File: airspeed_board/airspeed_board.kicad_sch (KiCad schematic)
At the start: 6 parts, among them J1 BME280, J2 ADXL345, J3 MPXV5002DP, U1 ESP32-C3_SUPERMINI, U2 XGZP6897D_1, U3 XGZP6897D_2

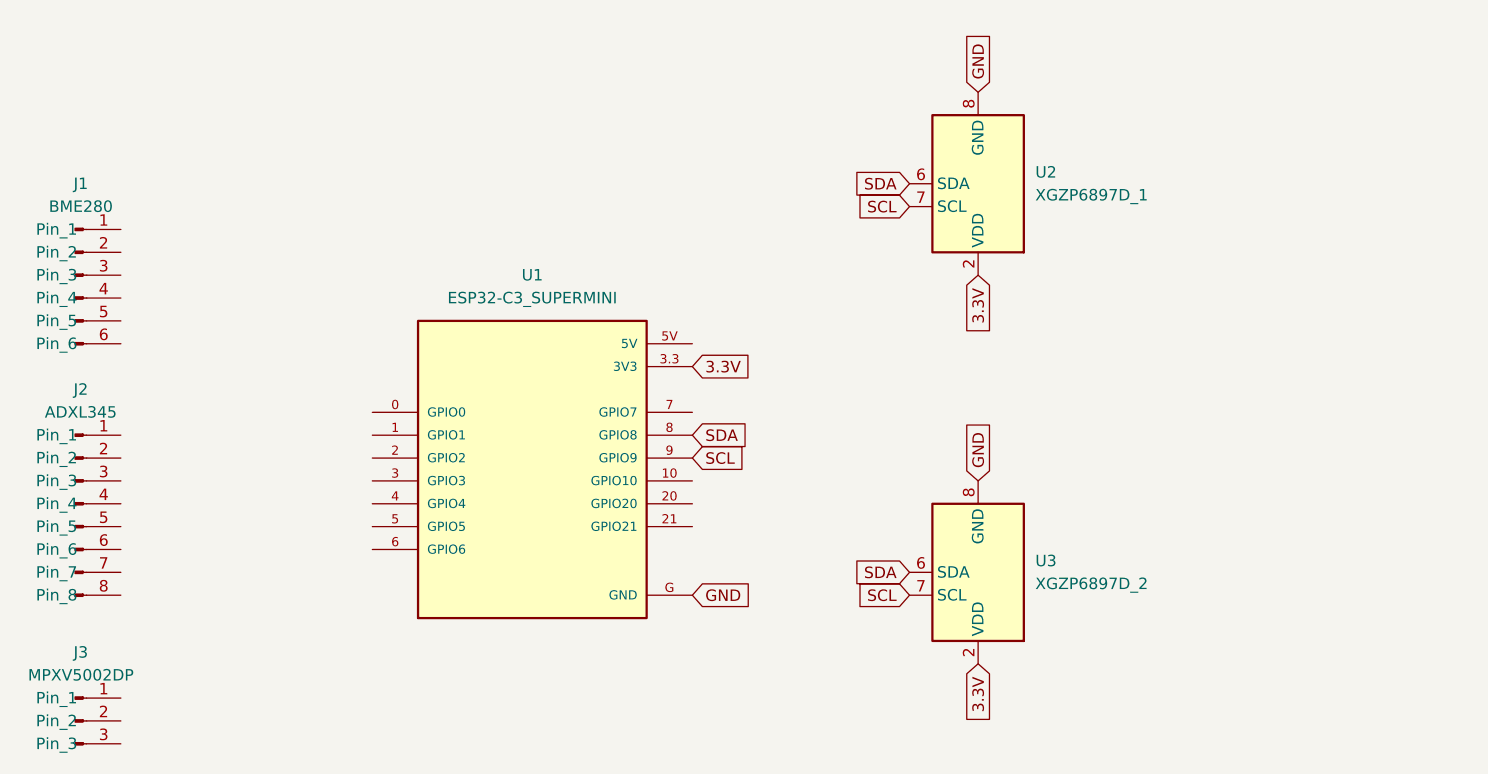
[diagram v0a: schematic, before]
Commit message: updated board layout
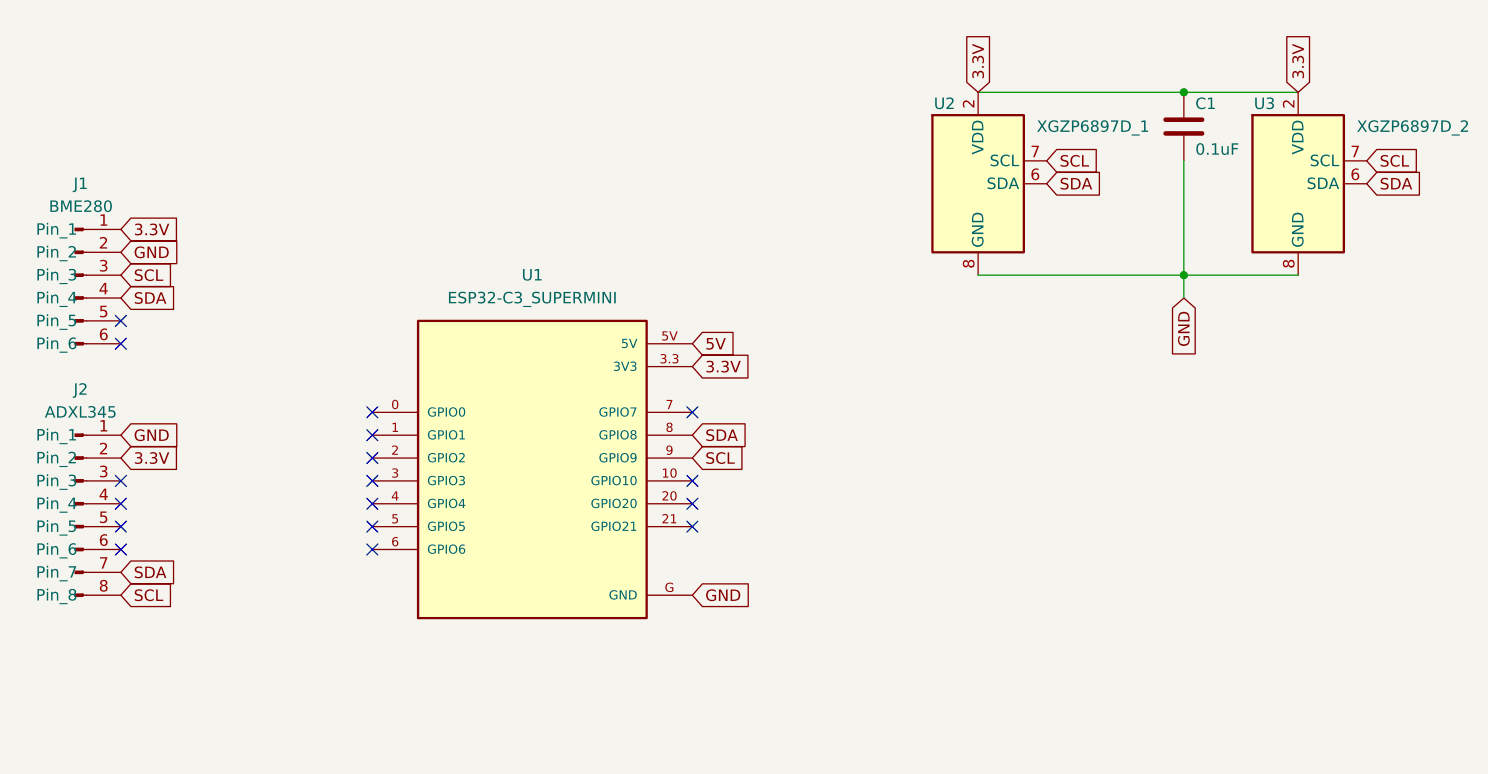
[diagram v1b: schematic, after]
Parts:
- removed J3: MPXV5002DP, Connector_PinHeader_2.54mm:PinHeader_1x03_P2.54mm_Vertical, symbol Connector:Conn_01x03_Pin
- added C1: 0.1uF, Capacitor_SMD:C_0805_2012Metric, symbol Device:C
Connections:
- net 3.3V: now also J1.1 (Pin_1), J2.2 (Pin_2), C1.2
- net GND: now also J1.2 (Pin_2), J2.1 (Pin_1), C1.1
- net SCL: now also J1.3 (Pin_3), J2.8 (Pin_8)
- net SDA: now also J1.4 (Pin_4), J2.7 (Pin_7)
- net 5V: now reaches U1.5V
- no-connect marks 0 -> 17
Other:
- moved on the sheet: U2

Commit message: updates to pcb
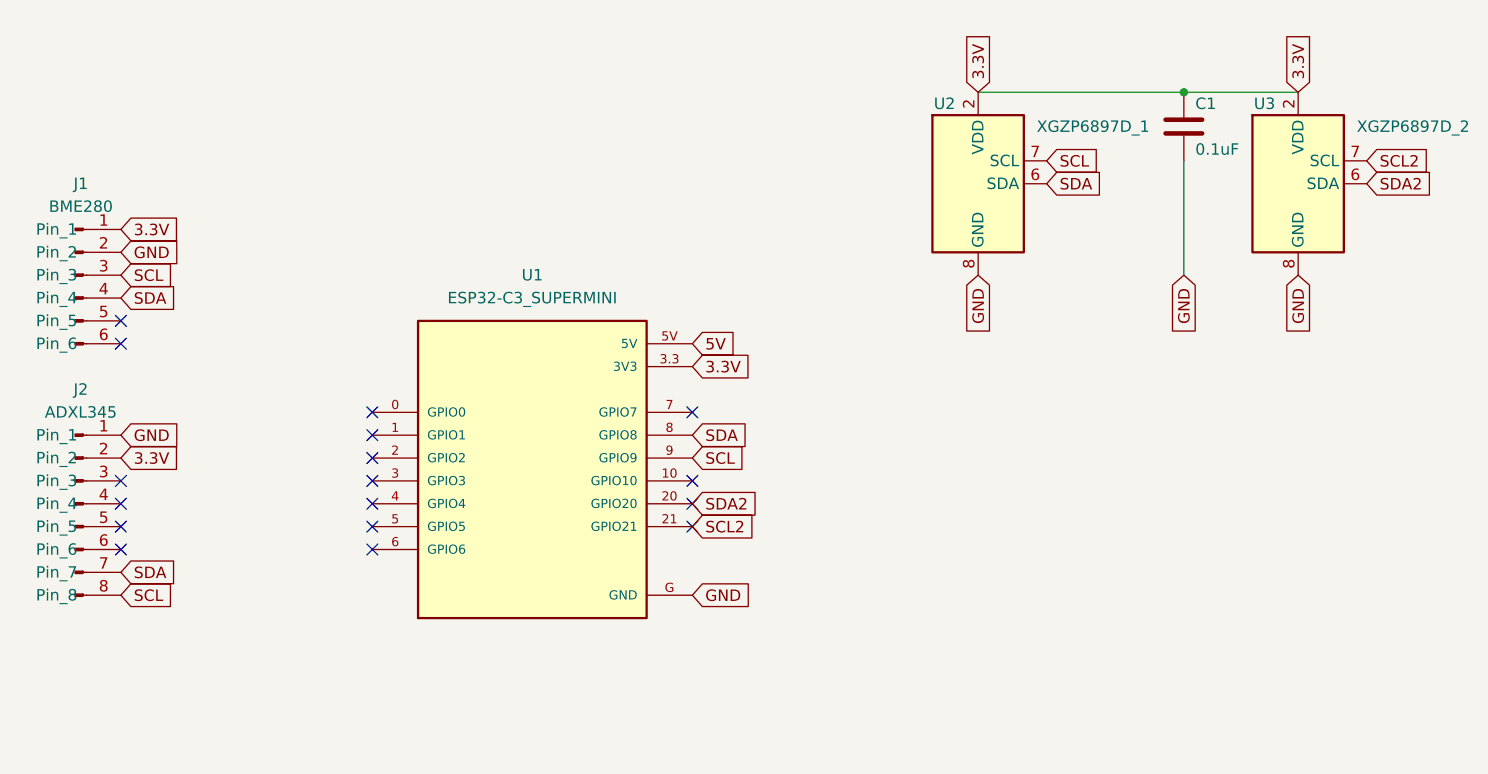
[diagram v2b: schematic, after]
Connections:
- net SCL: no longer U3.7 (SCL)
- net SDA: no longer U3.6 (SDA)
- net SDA2: now reaches U1.20 (GPIO20)
- net SDA2: now also U3.6 (SDA)
- net SCL2: now reaches U1.21 (GPIO21)
- net SCL2: now also U3.7 (SCL)
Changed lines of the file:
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@@
   (junction (at 193.04 36.83) (diameter 0) (color 0 0 0 0)
-  )
-  (junction (at 193.04 57.15) (diameter 0) (color 0 0 0 0)
   )
   (no_connect (at 102.87 77.47))
@@
   (no_connect (at 138.43 82.55))
   (no_connect (at 74.93 87.63))
-  (wire (pts (xy 170.18 57.15) (xy 193.04 57.15))
-    (stroke (width 0) (type default))
-  )
   (wire (pts (xy 193.04 57.15) (xy 193.04 44.45))
     (stroke (width 0) (type default))
   )
   (wire (pts (xy 193.04 36.83) (xy 205.74 36.83))
-    (stroke (width 0) (type default))
-  )
-  (wire (pts (xy 193.04 59.69) (xy 193.04 57.15))
-    (stroke (width 0) (type default))
-  )
-  (wire (pts (xy 193.04 57.15) (xy 205.74 57.15))
     (stroke (width 0) (type default))
   )
@@
     )
   )
-  (global_label "SDA" (shape input) (at 213.36 46.99 0) (fields_autoplaced)
+  (global_label "SDA2" (shape input) (at 213.36 46.99 0) (fields_autoplaced)
     (effects (font (size 1.27 1.27)) (justify left))
-    (property "Intersheetrefs" "${INTERSHEET_REFS}" (at 219.9133 46.99 0)
+    (property "Intersheetrefs" "${INTERSHEET_REFS}" (at 221.1228 46.99 0)
       (effects (font (size 1.27 1.27)) (justify left) hide)
     )
@@
     )
   )
-  (global_label "SCL" (shape input) (at 213.36 44.45 0) (fields_autoplaced)
+  (global_label "SCL2" (shape input) (at 213.36 44.45 0) (fields_autoplaced)
     (effects (font (size 1.27 1.27)) (justify left))
-    (property "Intersheetrefs" "${INTERSHEET_REFS}" (at 219.8528 44.45 0)
+    (property "Intersheetrefs" "${INTERSHEET_REFS}" (at 221.0623 44.45 0)
       (effects (font (size 1.27 1.27)) (justify left) hide)
     )
@@
     (effects (font (size 1.27 1.27)) (justify left))
     (property "Intersheetrefs" "${INTERSHEET_REFS}" (at 184.3533 46.99 0)
+      (effects (font (size 1.27 1.27)) (justify left) hide)
+    )
+  )
+  (global_label "SCL2" (shape input) (at 138.43 85.09 0) (fields_autoplaced)
+    (effects (font (size 1.27 1.27)) (justify left))
+    (property "Intersheetrefs" "${INTERSHEET_REFS}" (at 146.1323 85.09 0)
       (effects (font (size 1.27 1.27)) (justify left) hide)
     )
@@
     )
   )
+  (global_label "SDA2" (shape input) (at 138.43 82.55 0) (fields_autoplaced)
+    (effects (font (size 1.27 1.27)) (justify left))
+    (property "Intersheetrefs" "${INTERSHEET_REFS}" (at 146.1928 82.55 0)
+      (effects (font (size 1.27 1.27)) (justify left) hide)
+    )
+  )
   (global_label "SCL" (shape input) (at 74.93 92.71 0) (fields_autoplaced)
     (effects (font (size 1.27 1.27)) (justify left))
@@
     )
   )
+  (global_label "GND" (shape input) (at 193.04 57.15 270) (fields_autoplaced)
+    (effects (font (size 1.27 1.27)) (justify right))
+    (property "Intersheetrefs" "${INTERSHEET_REFS}" (at 193.04 64.0057 90)
+      (effects (font (size 1.27 1.27)) (justify right) hide)
+    )
+  )
   (global_label "GND" (shape input) (at 74.93 54.61 0) (fields_autoplaced)
     (effects (font (size 1.27 1.27)) (justify left))
     (property "Intersheetrefs" "${INTERSHEET_REFS}" (at 81.7857 54.61 0)
       (effects (font (size 1.27 1.27)) (justify left) hide)
+    )
+  )
+  (global_label "GND" (shape input) (at 205.74 57.15 270) (fields_autoplaced)
+    (effects (font (size 1.27 1.27)) (justify right))
+    (property "Intersheetrefs" "${INTERSHEET_REFS}" (at 205.74 64.0057 90)
+      (effects (font (size 1.27 1.27)) (justify right) hide)
     )
   )
@@
     )
   )
-  (global_label "GND" (shape input) (at 193.04 59.69 270) (fields_autoplaced)
+  (global_label "GND" (shape input) (at 170.18 57.15 270) (fields_autoplaced)
     (effects (font (size 1.27 1.27)) (justify right))
-    (property "Intersheetrefs" "${INTERSHEET_REFS}" (at 193.04 66.5457 90)
+    (property "Intersheetrefs" "${INTERSHEET_REFS}" (at 170.18 64.0057 90)
       (effects (font (size 1.27 1.27)) (justify right) hide)
     )
